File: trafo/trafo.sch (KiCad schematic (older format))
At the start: 16 parts

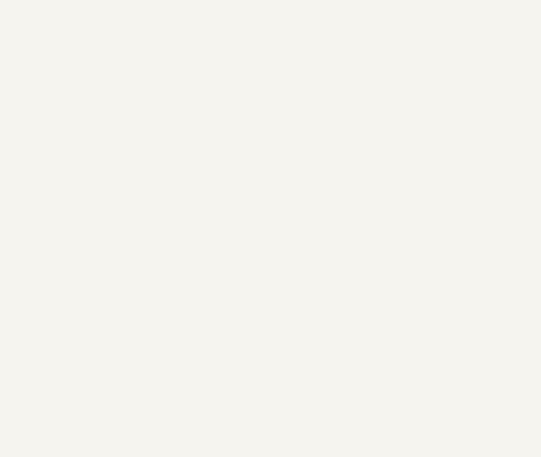
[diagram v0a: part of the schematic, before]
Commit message: added overview
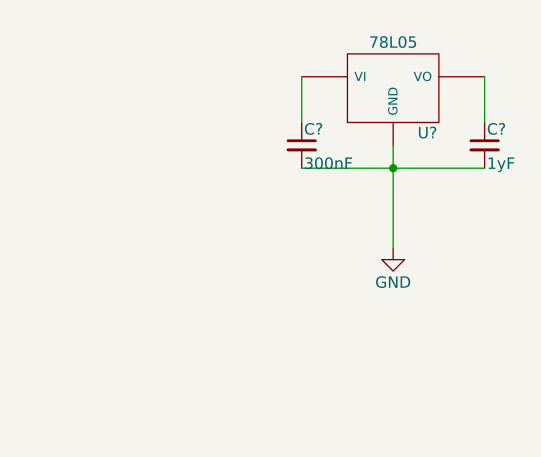
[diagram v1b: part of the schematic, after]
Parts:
- added C?: 300nF, symbol C_Small
- added C?: 1yF, symbol C_Small
- added U?: 78L05, symbol 78L05
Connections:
- net GND: now also C?.2, C?.2, U?.GND
- new net: C?.1, U?.VI
- new net: C?.1, U?.VO
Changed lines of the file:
@@
 Wire Wire Line
 	3800 5500 3400 5500
+$Comp
+L 78L05 U?
+U 1 1 5AAED6FB
+P 8950 1250
+F 0 "U?" H 9100 1054 50  0000 C CNN
+F 1 "78L05" H 8950 1450 50  0000 C CNN
+F 2 "" H 8950 1250 50  0000 C CNN
+F 3 "" H 8950 1250 50  0000 C CNN
+	1    8950 1250
+	1    0    0    -1
+$EndComp
+$Comp
+L C_Small C?
+U 1 1 5AAEDC89
+P 8550 1500
+F 0 "C?" H 8560 1570 50  0000 L CNN
+F 1 "300nF" H 8560 1420 50  0000 L CNN
+F 2 "" H 8550 1500 50  0000 C CNN
+F 3 "" H 8550 1500 50  0000 C CNN
+	1    8550 1500
+	1    0    0    -1
+$EndComp
+$Comp
+L C_Small C?
+U 1 1 5AAEDD00
+P 9350 1500
+F 0 "C?" H 9360 1570 50  0000 L CNN
+F 1 "1yF" H 9360 1420 50  0000 L CNN
+F 2 "" H 9350 1500 50  0000 C CNN
+F 3 "" H 9350 1500 50  0000 C CNN
+	1    9350 1500
+	1    0    0    -1
+$EndComp
+$Comp
+L GND #PWR?
+U 1 1 5AAEDD5C
+P 8950 1950
+F 0 "#PWR?" H 8950 1700 50  0001 C CNN
+F 1 "GND" H 8950 1800 50  0000 C CNN
+F 2 "" H 8950 1950 50  0000 C CNN
+F 3 "" H 8950 1950 50  0000 C CNN
+	1    8950 1950
+	1    0    0    -1
+$EndComp
+Wire Wire Line
+	8950 1500 8950 1950
+Wire Wire Line
+	8550 1400 8550 1200
+Wire Wire Line
+	8550 1600 9350 1600
+Connection ~ 8950 1600
+Wire Wire Line
+	9350 1400 9350 1200
 $EndSCHEMATC
